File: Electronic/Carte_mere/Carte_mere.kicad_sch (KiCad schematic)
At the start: 64 parts, among them J1 USB_C_Receptacle_USB2.0_14P, J10 Conn_01x07, J11 Conn_01x08, J2 Conn_01x04, J3 Conn_01x02, J4 Conn_01x02, J5 Conn_01x07, J6 Conn_01x07, J7 xt60pm, J8 Conn_01x11, J9 Conn_01x07, SW1 push button, SW2 push button RST, U1 TPS5431DDA, U2 ESP32-S3-WROOM-2, U3 TPS5431DDA

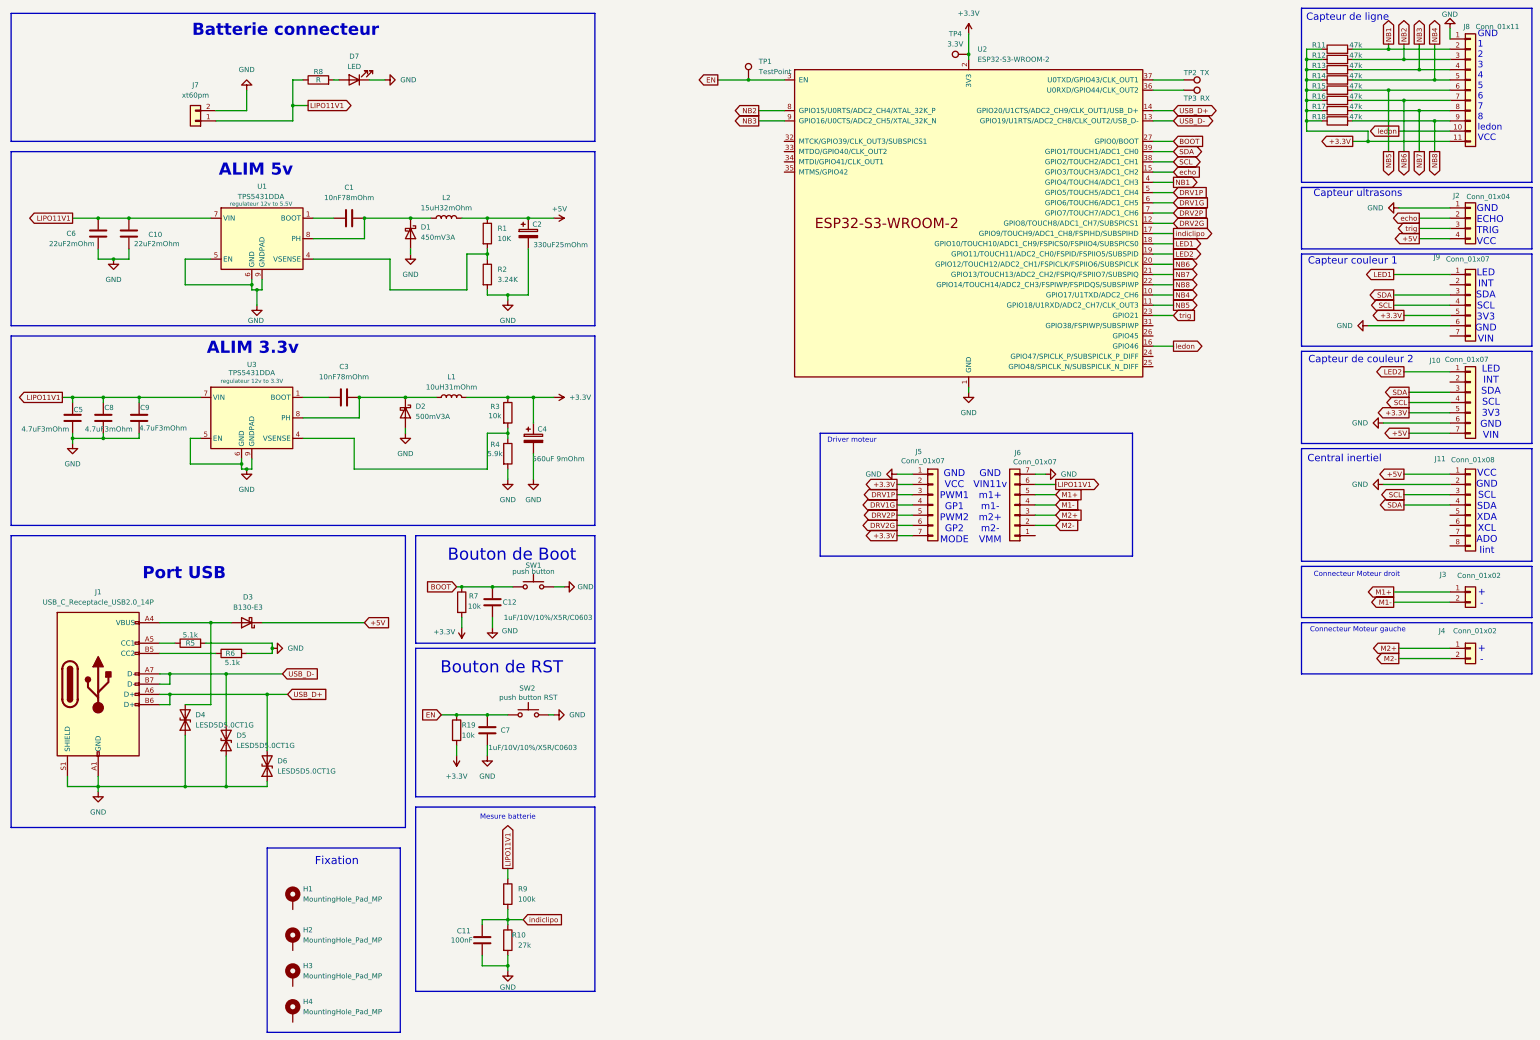
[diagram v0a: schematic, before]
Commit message: Add files via upload
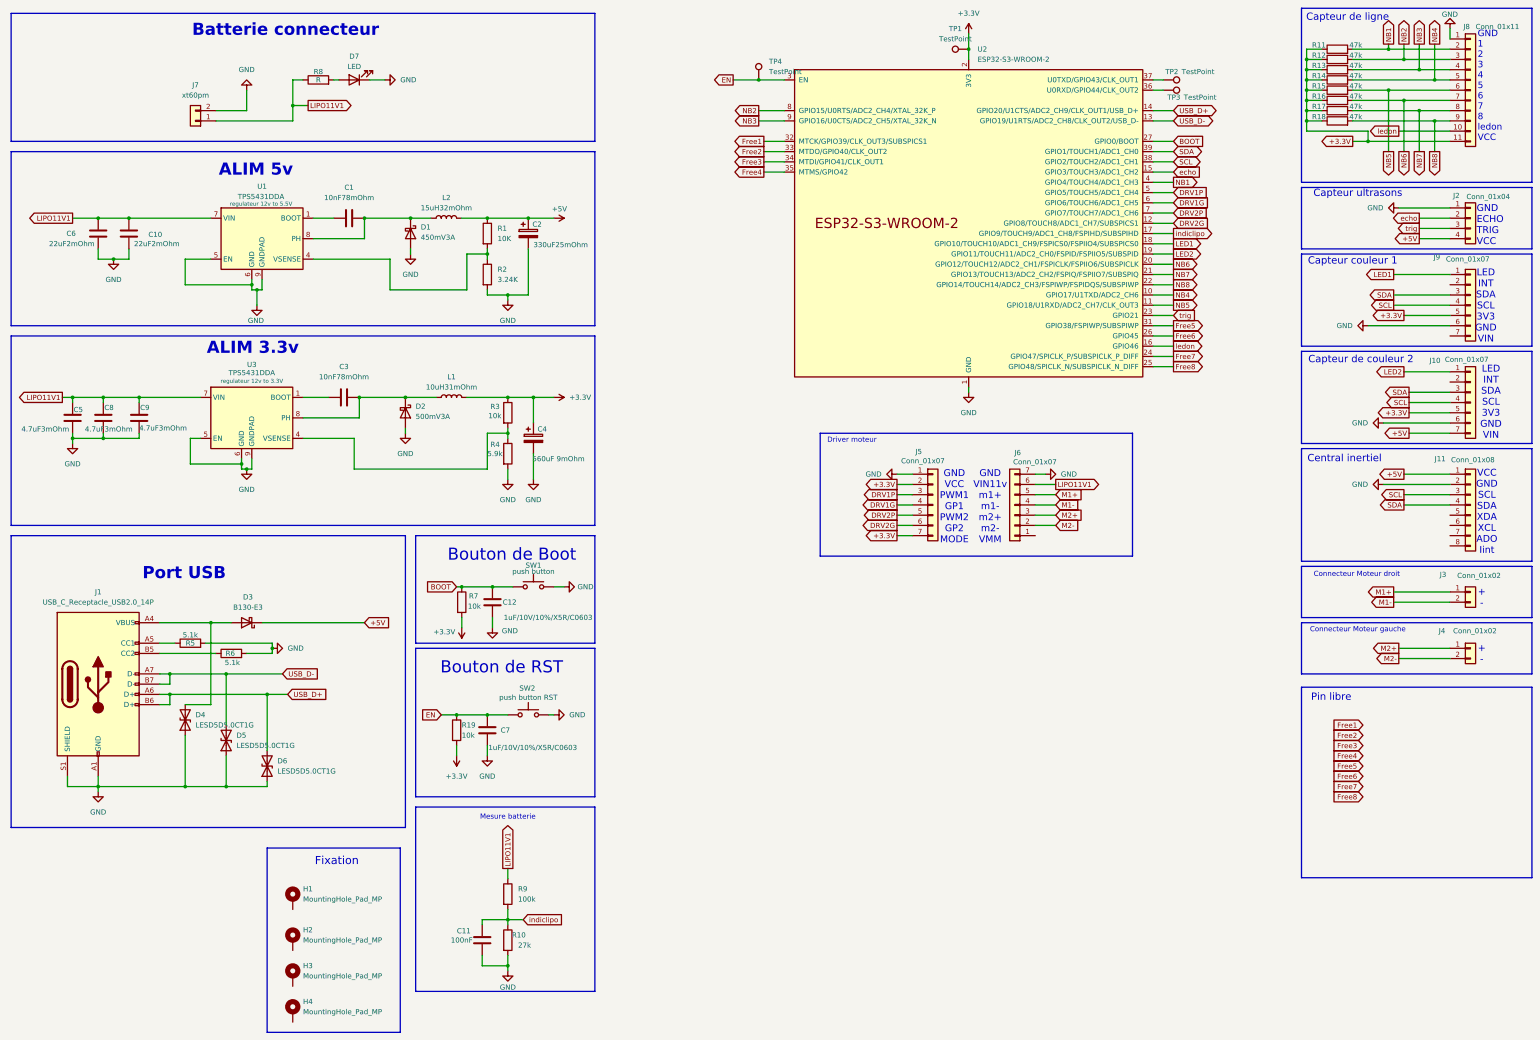
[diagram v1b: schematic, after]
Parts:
- TP2: value TX -> TestPoint
- TP3: value RX -> TestPoint
- TP4: value 3.3V -> TestPoint
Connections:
- net +3.3V: now also TP1.1; no longer TP4.1
- net EN: now also TP4.1; no longer TP1.1
- net Free7: now reaches U2.24 (GPIO47/SPICLK_P/SUBSPICLK_P_DIFF)
- net Free8: now reaches U2.25 (GPIO48/SPICLK_N/SUBSPICLK_N_DIFF)
- net Free6: now reaches U2.26 (GPIO45)
- net Free5: now reaches U2.31 (GPIO38/FSPIWP/SUBSPIWP)
- net Free1: now reaches U2.32 (MTCK/GPIO39/CLK_OUT3/SUBSPICS1)
- net Free2: now reaches U2.33 (MTDO/GPIO40/CLK_OUT2)
- net Free3: now reaches U2.34 (MTDI/GPIO41/CLK_OUT1)
- net Free4: now reaches U2.35 (MTMS/GPIO42)
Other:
- note added: "Pin libre"
